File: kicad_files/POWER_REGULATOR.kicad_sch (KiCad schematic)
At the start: 35 parts, among them IC2 LTC3569EUDC#PBF, IC3 MBT3904DW1T1G, Q1 SI2302CDS-T1-E3, Q2 MMBT4403LT3G

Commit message: pcb layout updated
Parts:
- L1, L2, L3: footprint (none) -> Inductor_SMD:L_0805_2012Metric
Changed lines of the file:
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@@
       (effects (font (size 1.27 1.27)))
     )
-    (property "Footprint" "" (at 141.605 75.565 0)
+    (property "Footprint" "Inductor_SMD:L_0805_2012Metric" (at 141.605 75.565 0)
       (effects (font (size 1.27 1.27)) hide)
     )
@@
       (effects (font (size 1.27 1.27)))
     )
-    (property "Footprint" "" (at 141.605 57.15 0)
+    (property "Footprint" "Inductor_SMD:L_0805_2012Metric" (at 141.605 57.15 0)
       (effects (font (size 1.27 1.27)) hide)
     )
@@
       (effects (font (size 1.27 1.27)))
     )
-    (property "Footprint" "" (at 141.605 66.04 0)
-      (effects (font (size 1.27 1.27)) hide)
-    )
+    (property "Footprint" "Inductor_SMD:L_0805_2012Metric" (at 141.605 66.04 0)
+      (effects (font (size 1.27 1.27)) hide)
+    )

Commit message: layout basic completed
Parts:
- C45, C48: footprint Capacitor_SMD:C_0402_1005Metric_Pad0.74x0.62mm_HandSolder -> Capacitor_SMD:C_0805_2012Metric_Pad1.18x1.45mm_HandSolder
- C50, C52: footprint Capacitor_SMD:C_0402_1005Metric_Pad0.74x0.62mm_HandSolder -> Capacitor_SMD:C_0603_1608Metric_Pad1.08x0.95mm_HandSolder
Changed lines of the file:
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@@
       (effects (font (size 1.27 1.27)) (justify left))
     )
-    (property "Footprint" "Capacitor_SMD:C_0402_1005Metric_Pad0.74x0.62mm_HandSolder" (at 88.9 42.545 0)
+    (property "Footprint" "Capacitor_SMD:C_0805_2012Metric_Pad1.18x1.45mm_HandSolder" (at 88.9 42.545 0)
       (effects (font (size 1.27 1.27)) hide)
     )
@@
       (effects (font (size 1.27 1.27)) (justify left))
     )
-    (property "Footprint" "Capacitor_SMD:C_0402_1005Metric_Pad0.74x0.62mm_HandSolder" (at 170.18 60.325 0)
+    (property "Footprint" "Capacitor_SMD:C_0805_2012Metric_Pad1.18x1.45mm_HandSolder" (at 170.18 60.325 0)
       (effects (font (size 1.27 1.27)) hide)
     )
@@
       (effects (font (size 1.27 1.27)) (justify left))
     )
-    (property "Footprint" "Capacitor_SMD:C_0402_1005Metric_Pad0.74x0.62mm_HandSolder" (at 170.18 69.215 0)
+    (property "Footprint" "Capacitor_SMD:C_0603_1608Metric_Pad1.08x0.95mm_HandSolder" (at 170.18 69.215 0)
       (effects (font (size 1.27 1.27)) hide)
     )
@@
       (effects (font (size 1.27 1.27)) (justify left))
     )
-    (property "Footprint" "Capacitor_SMD:C_0402_1005Metric_Pad0.74x0.62mm_HandSolder" (at 170.18 78.74 0)
-      (effects (font (size 1.27 1.27)) hide)
-    )
+    (property "Footprint" "Capacitor_SMD:C_0603_1608Metric_Pad1.08x0.95mm_HandSolder" (at 170.18 78.74 0)
+      (effects (font (size 1.27 1.27)) hide)
+    )

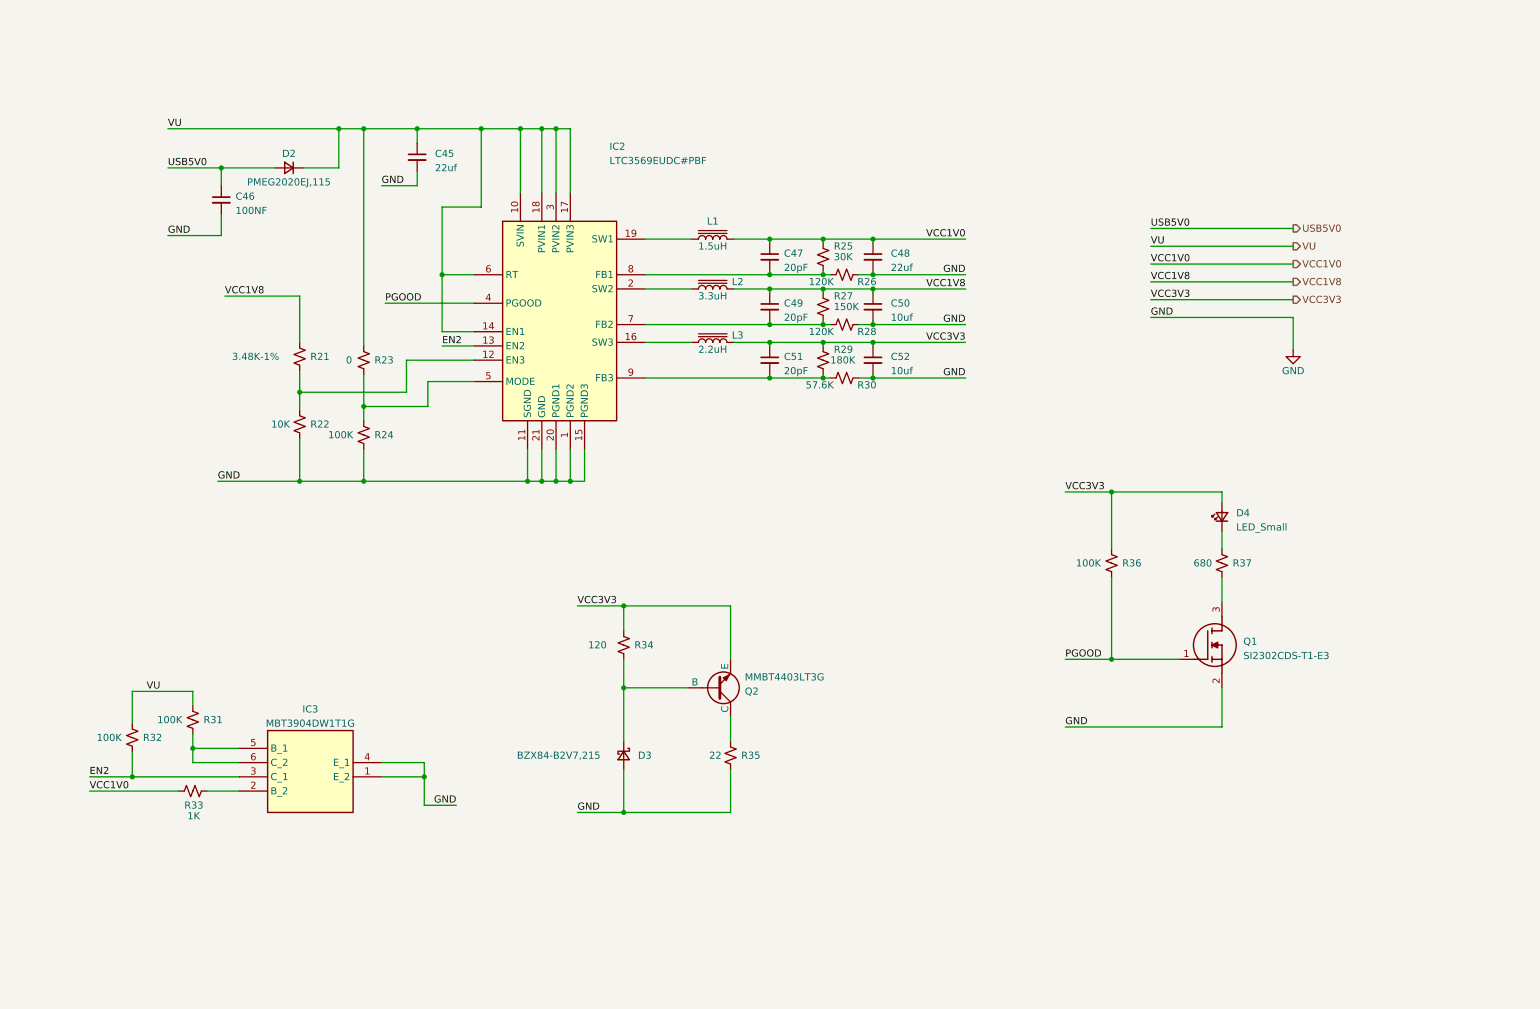
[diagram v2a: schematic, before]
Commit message: updated files
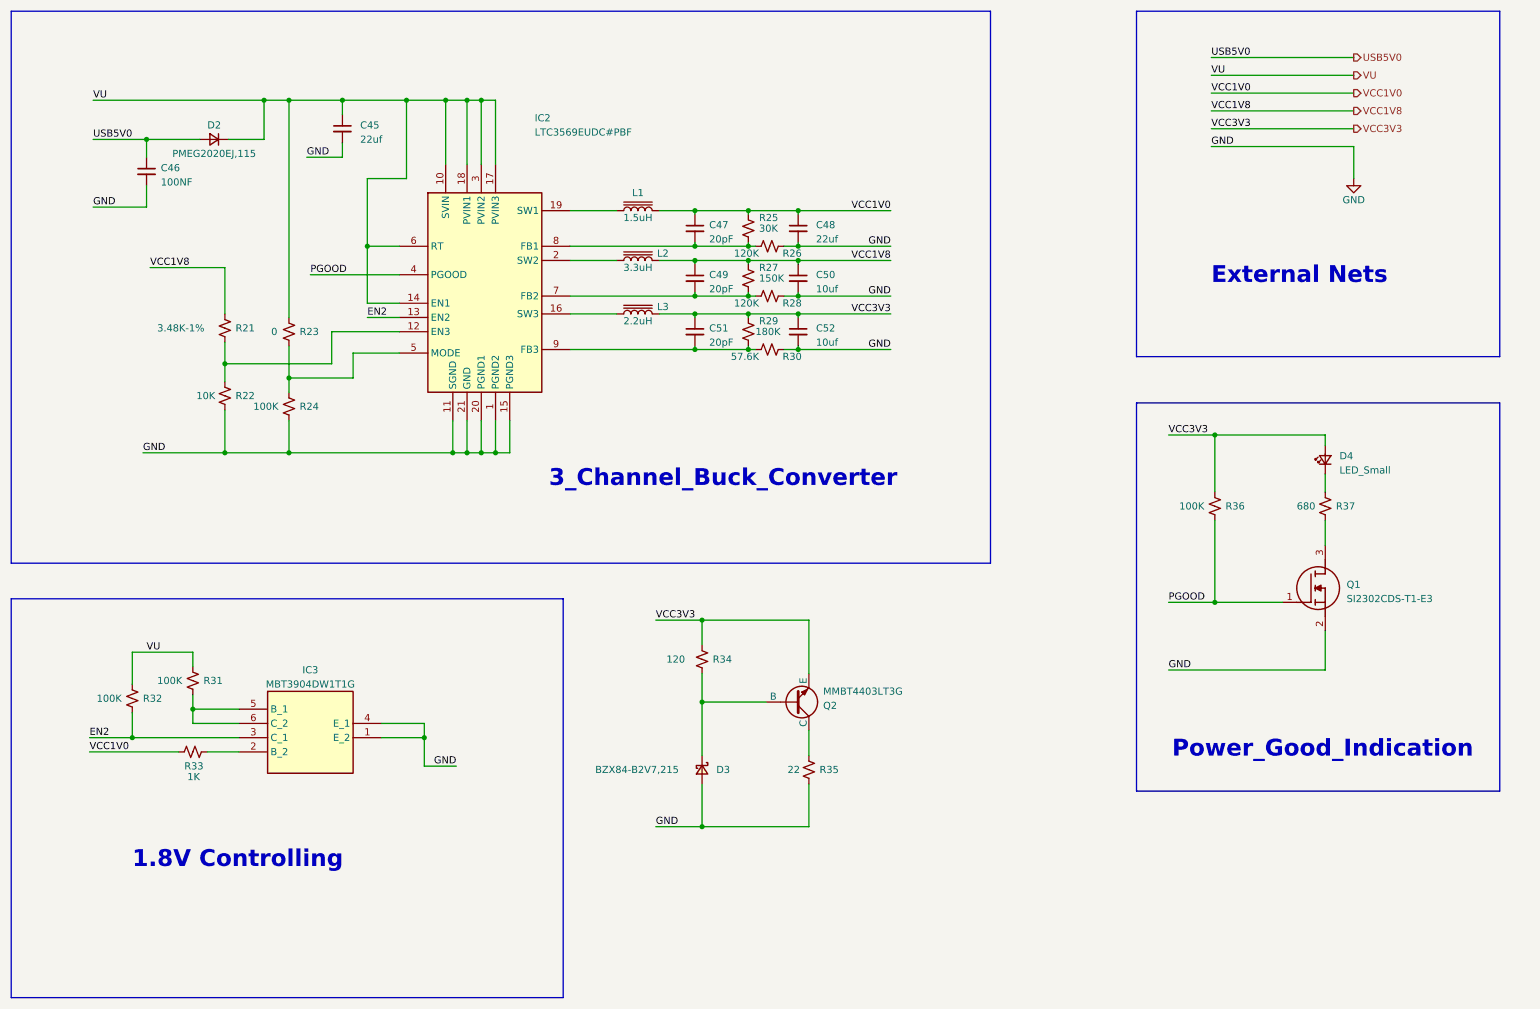
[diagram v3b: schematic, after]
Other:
- note added: "1.8V Controlling"
- note added: "3_Channel_Buck_Converter"
- note added: "External Nets"
- note added: "Power_Good_Indication"
- moved on the sheet: C45, C46, C47, C48, C49, C50, C51, C52, D2, D3, D4, IC2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
